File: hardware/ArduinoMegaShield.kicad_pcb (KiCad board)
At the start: 2 copper layers, 41 parts, among them J201 DB15, J202 DB9, J203 DB9, P201 CONN_01X02, P202 CONN_01X08, P203 CONN_01X08, P204 CONN_01X02, SW101 SW_Coded, SW102 SW_Coded, SW103 SW_Coded, U101 A4988, U102 A4988, U103 A4988

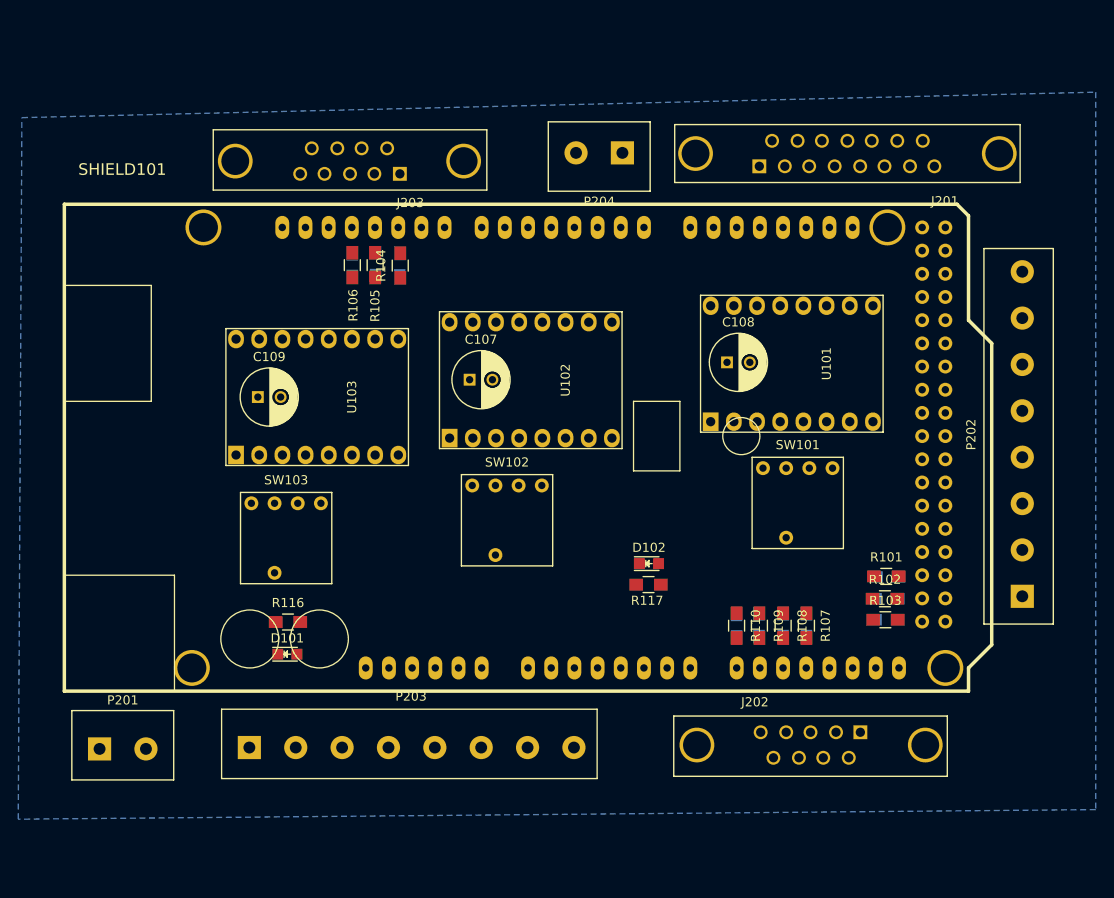
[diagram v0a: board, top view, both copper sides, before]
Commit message: completed board and generated gerbers
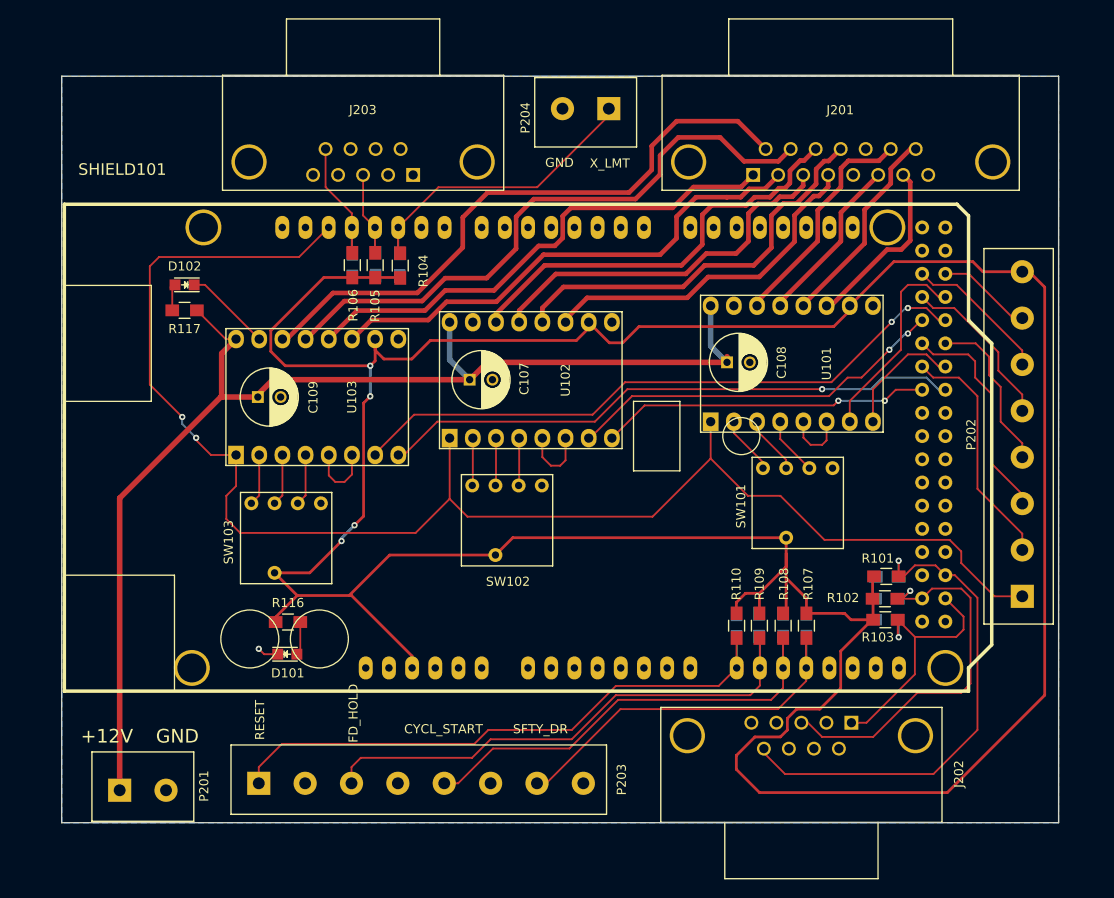
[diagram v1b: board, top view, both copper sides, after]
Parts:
- J201: footprint Connectors:DB15FD -> 6axis:D15S33E4GV00LF
- J202: footprint Connectors:DB9FD -> 6axis:LD09S33E4GV00LF
- J203: footprint Connectors:DB9MD -> 6axis:LD09P33E4GV00LF
- moved D102 59.3 mm to (87.1, 89.4), turned to 180 degrees
- moved R117 59.0 mm to (87.1, 92.2), turned to 180 degrees
- moved P204 5.07 mm to (131.1, 70.1)
- moved P201 5.04 mm to (82.5, 144.8)
- moved P203 4.05 mm to (113.0, 144.0)
- moved J202 1.52 mm to (154.7, 138.8), turned to 180 degrees
- moved J201 1.48 mm to (159.0, 75.9), turned to 0 degrees
- moved J203 1.43 mm to (106.7, 75.9), turned to 0 degrees
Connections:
- J201 pad 1: /C2B -> /C1A
- J201 pad 10: /C1A -> /C2A
- J201 pad 11: /B2A -> /B2B
- J201 pad 12: /B1B -> /B1A
- J201 pad 14: /A2A -> /A2B
- J201 pad 15: /A1B -> /A1A
- J201 pad 3: /B2B -> /B2A
- J201 pad 4: GND -> /B1B
- J201 pad 5: /B1A -> GND
- J201 pad 6: /A2B -> /A2A
- J201 pad 7: GND -> /A1B
- J201 pad 8: /A1A -> GND
- J201 pad 9: /C2A -> /C2B
- P202 pad 3: /~Y-Dir -> /~X-Dir
- P202 pad 4: /~X-Dir -> /~Y-Dir
- P202 pad 6: /~Y-Step -> /~X-Step
- P202 pad 7: /~X-Step -> /~Y-Step
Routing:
- net +5V: track 0.00 -> 368.0 mm, vias 0 -> 4
- net /~ENABLE: track 0.00 -> 165.5 mm, vias 0 -> 2
- net +12V: track 0.00 -> 132.2 mm
- net /C-Step: track 0.00 -> 69.8 mm, vias 0 -> 2
- net /C2B: track 0.00 -> 67.6 mm
- net /C2A: track 0.00 -> 67.2 mm
- net /RESET: track 0.00 -> 65.3 mm
- net /C-Dir: track 0.00 -> 64.0 mm, vias 0 -> 1
- net /FEED_HOLD: track 0.00 -> 58.9 mm
- net /C_LIMIT: track 0.00 -> 55.9 mm, vias 0 -> 1
- net /C1B: track 0.00 -> 55.6 mm
- net /C1A: track 0.00 -> 55.4 mm
- net /CYCLE_START: track 0.00 -> 50.4 mm
- net /B2B: track 0.00 -> 46.2 mm
- net /B1A: track 0.00 -> 44.5 mm
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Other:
- board outline added: 109.2 x 81.8 mm
- net class Default: clearance 0.1524 -> 0.2032
- rule trace_clearance: 0.1524 -> 0.2032
- board text added: "+12V"
- board text added: "6-Axis Robot Arm Control Shield Designed By: Alan Ford David Andra Bruce Davies"
- board text added: "CYCL_START"
- board text added: "FD_HOLD"
- board text added: "GND"
- board text added: "RESET"
- board text added: "SFTY_DR"
- board text added: "X_LMT"
